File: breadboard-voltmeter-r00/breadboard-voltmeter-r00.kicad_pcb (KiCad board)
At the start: 2 copper layers, 12 x 19.4 mm, 11 parts, among them J1 OLED_display, J2 Power_supply, J3 Conn_01x03_Pin, U1 CH32V003J4M6

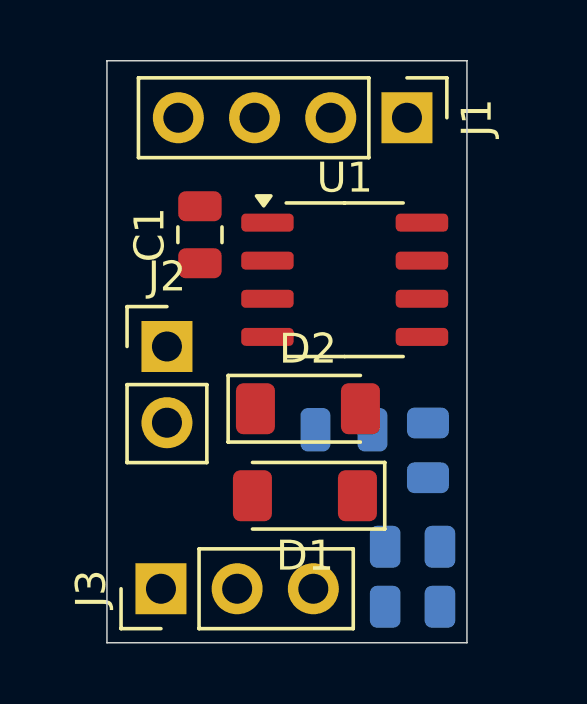
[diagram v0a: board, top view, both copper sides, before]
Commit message: finished design, ready to production
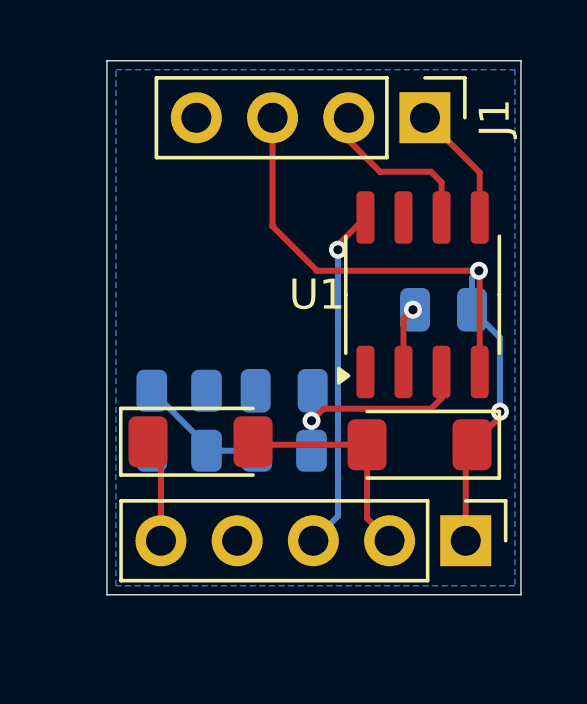
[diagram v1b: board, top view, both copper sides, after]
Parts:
- removed J3: Conn_01x03_Pin, Connector_PinHeader_2.54mm:PinHeader_1x03_P2.54mm_Vertical
- C1: moved to B.Cu
- J2: value Power_supply -> Conn_01x05_Pin; footprint Connector_PinHeader_2.54mm:PinHeader_1x02_P2.54mm_Vertical -> Connector_PinHeader_2.54mm:PinHeader_1x05_P2.54mm_Vertical
- moved J2 11.9 mm to (133.0, 61.1), turned to -90 degrees
- moved R1 9.36 mm to (123.4, 58.1)
- moved R2 9.36 mm to (123.4, 56.1), turned to 0 degrees
- moved C1 8.50 mm to (132.2, 53.4), turned to 180 degrees
- moved R3 4.79 mm to (126.9, 58.1), turned to 0 degrees
- moved D1 3.92 mm to (124.1, 57.8), turned to 0 degrees
- moved D2 3.91 mm to (131.4, 57.9), turned to 180 degrees
- moved U1 2.64 mm to (131.5, 52.9), turned to 90 degrees
- moved C2 2.38 mm to (126.9, 56.1)
- moved J1 0.60 mm to (131.6, 47.0)
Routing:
- net PowerSupply: track 0.00 -> 24.5 mm, vias 0 -> 2
- net SWIO: track 0.00 -> 11.5 mm, vias 0 -> 1
- net GND: track 0.00 -> 9.56 mm, vias 0 -> 1
- net Voltage: track 0.00 -> 7.62 mm, vias 0 -> 1
- net Net-(D1-K): track 0.00 -> 6.60 mm
- net SCL: track 0.00 -> 5.60 mm
- net Net-(R1-Pad2): track 0.00 -> 4.43 mm
- net SDA: track 0.00 -> 4.08 mm
- added copper zone on B.Cu, net GND
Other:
- board size 12 x 19.4 mm -> 13.8 x 17.8 mm
- board text added: "FritzenLab.net CH32V003 voltmeter"

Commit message: edited schematics
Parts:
- R1: value 82000 -> 68000
- R2: value 15000 -> 12000
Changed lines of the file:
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@@
 		(tags "Diode Mini-MELF (SOD-80)")
 		(property "Reference" "D1"
-			(at 0.1875 0.7 360)
+			(at 0.1875 0.7 0)
 			(layer "F.SilkS")
 			(hide yes)
@@
 		)
 		(property "Value" "D"
-			(at 0 2 360)
+			(at 0 2 0)
 			(layer "F.Fab")
 			(hide yes)
@@
 		(tags "Diode Mini-MELF (SOD-80)")
 		(property "Reference" "D2"
-			(at 0 0 360)
+			(at 0 0 0)
 			(layer "F.SilkS")
 			(hide yes)
@@
 		)
 		(property "Value" "D"
-			(at 0 2 360)
+			(at 0 2 0)
 			(layer "F.Fab")
 			(effects
@@
 		(tags "resistor")
 		(property "Reference" "R3"
-			(at -0.1075 1.4 360)
+			(at -0.1075 1.4 0)
 			(layer "B.SilkS")
 			(hide yes)
@@
 		)
 		(property "Value" "4700"
-			(at 0 -1.65 360)
+			(at 0 -1.65 0)
 			(layer "B.Fab")
 			(hide yes)
@@
 		)
 		(fp_text user "${REFERENCE}"
-			(at 0 0 360)
+			(at 0 0 0)
 			(layer "B.Fab")
 			(effects
@@
 		(tags "capacitor")
 		(property "Reference" "C1"
-			(at 2.62 0 360)
+			(at 2.62 0 0)
 			(layer "B.SilkS")
 			(effects
@@
 		)
 		(property "Value" "100n"
-			(at 0 -1.68 360)
+			(at 0 -1.68 0)
 			(layer "B.Fab")
 			(hide yes)
@@
 		)
 		(fp_text user "${REFERENCE}"
-			(at -0.9 0.2 360)
+			(at -0.9 0.2 0)
 			(layer "B.Fab")
 			(effects
@@
 		(tags "resistor")
 		(property "Reference" "R2"
-			(at 0.1925 -1.7 360)
+			(at 0.1925 -1.7 0)
 			(layer "B.SilkS")
 			(effects
@@
 			)
 		)
-		(property "Value" "15000"
-			(at 0 -1.65 360)
+		(property "Value" "12000"
+			(at 0 -1.65 0)
 			(layer "B.Fab")
 			(hide yes)
@@
 		)
 		(fp_text user "${REFERENCE}"
-			(at 0 0 360)
+			(at 0 0 0)
 			(layer "B.Fab")
 			(effects
@@
 			)
 		)
-		(property "Value" "82000"
+		(property "Value" "68000"
 			(at 0 -1.65 0)
 			(layer "B.Fab")
